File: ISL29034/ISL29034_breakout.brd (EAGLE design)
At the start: 15.2 x 11.2 mm, 2 parts

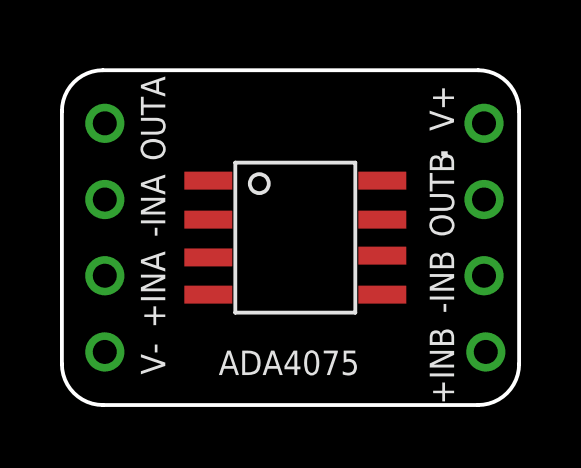
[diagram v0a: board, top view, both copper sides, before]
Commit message: Update new meme.
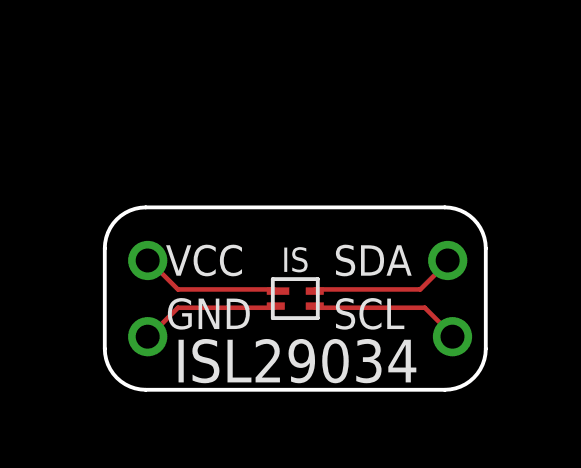
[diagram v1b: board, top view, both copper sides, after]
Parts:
- removed .: ADA4075, FaBo-Opamp:SOIC(NARROW)-8
- removed U$3: 8PIN, FaBo-Breakout:8PIN
- added IS: IN-ISL29034, FaBo-Mems:INTERSIL-ISL29034
- added U$1: 4PIN, FaBo-Breakout:4PIN
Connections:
- removed net 1: ..1, U$3.1
- removed net 2: ..2, U$3.2
- removed net 3: ..3, U$3.3
- removed net 4: ..4, U$3.4
- removed net 5: ..5, U$3.5
- removed net 6: ..6, U$3.6
- removed net 7: ..7, U$3.7
- removed net 8: ..8, U$3.8
- new net GND: IS.2, U$1.2
- new net SCL: IS.3, U$1.3
- new net SDA: IS.4, U$1.4
- new net VCC: IS.1, U$1.1
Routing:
- net SCL: track 0.00 -> 5.06 mm
- net SDA: track 0.00 -> 4.90 mm
- net VCC: track 0.00 -> 4.75 mm
- net GND: track 0.00 -> 4.68 mm
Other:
- board size 15.2 x 11.2 mm -> 12.7 x 6.1 mm
- board text added: "GND"
- board text added: "ISL29034"
- board text added: "SCL"
- board text added: "SDA"
- board text added: "VCC"
- board text removed: "+INA"
- board text removed: "+INB"
- board text removed: "-INA"
- board text removed: "-INB"
- board text removed: "ADA4075"
- board text removed: "OUTA"
- board text removed: "OUTB"
- board text removed: "V+"
- board text removed: "V-"
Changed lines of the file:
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@@
 <setting verticaltext="up"/>
 </settings>
-<grid distance="0.25" unitdist="mm" unit="mm" style="lines" multiple="1" display="yes" altdistance="0.025" altunitdist="inch" altunit="inch"/>
+<grid distance="0.01" unitdist="inch" unit="inch" style="lines" multiple="1" display="no" altdistance="0.025" altunitdist="inch" altunit="inch"/>
 <layers>
 <layer number="1" name="Top" color="4" fill="1" visible="yes" active="yes"/>
@@
 <layer number="49" name="Reference" color="7" fill="1" visible="yes" active="yes"/>
 <layer number="50" name="dxf" color="7" fill="1" visible="no" active="no"/>
-<layer number="51" name="tDocu" color="14" fill="1" visible="yes" active="yes"/>
+<layer number="51" name="tDocu" color="7" fill="1" visible="yes" active="yes"/>
 <layer number="52" name="bDocu" color="7" fill="1" visible="yes" active="yes"/>
 <layer number="53" name="tGND_GNDA" color="7" fill="9" visible="no" active="no"/>
@@
 <layer number="154" name="FabDoc2" color="2" fill="1" visible="no" active="no"/>
 <layer number="155" name="FabDoc3" color="7" fill="15" visible="no" active="no"/>
-<layer number="160" name="O_Dim" color="12" fill="11" visible="yes" active="yes"/>
 <layer number="199" name="Contour" color="7" fill="1" visible="yes" active="yes"/>
-<layer number="200" name="200bmp" color="1" fill="10" visible="yes" active="yes"/>
+<layer number="200" name="200bmp" color="1" fill="10" visible="no" active="yes"/>
 <layer number="201" name="201bmp" color="2" fill="1" visible="no" active="no"/>
 <layer number="202" name="202bmp" color="3" fill="1" visible="no" active="no"/>
@@
 <board>
 <plain>
-<text x="3.794" y="1.262" size="0.8128" layer="21">ADA4075</text>
-<text x="2.016" y="8.398" size="0.8128" layer="21" rot="R90">OUTA</text>
-<text x="2.016" y="5.858" size="0.8128" layer="21" rot="R90">-INA</text>
-<text x="2.016" y="2.818" size="0.8128" layer="21" rot="R90">+INA</text>
-<text x="11.64" y="9.398" size="0.8128" layer="21" rot="R90">V+</text>
-<text x="11.644" y="5.858" size="0.8128" layer="21" rot="R90">OUTB</text>
-<text x="11.644" y="3.318" size="0.8128" layer="21" rot="R90">-INB</text>
-<text x="11.644" y="0.278" size="0.8128" layer="21" rot="R90">+INB</text>
-<text x="2.016" y="1.278" size="0.8128" layer="21" rot="R90">V-</text>
+<text x="2.286" y="1.016" size="1.4224" layer="21">ISL29034</text>
+<text x="2.032" y="4.572" size="1.016" layer="21">VCC</text>
+<text x="2.032" y="2.794" size="1.016" layer="21">GND</text>
+<text x="7.62" y="4.572" size="1.016" layer="21">SDA</text>
+<text x="7.62" y="2.794" size="1.016" layer="21">SCL</text>
 </plain>
 <attributes>
@@
 </class>
 </classes>
-<designrules name="Elecrow_2-layer_eagle_rule">
+<designrules name="SeeedStudio_2layer_DRU_no_angle_20140221">
 <description language="de">&lt;b&gt;EAGLE Design Rules&lt;/b&gt;
 &lt;p&gt;
@@
 necessary adjustments and save your customized
 design rules under a new name.</description>
-<description language="zh">&lt;b&gt;Elecrow EAGLE Design Rules&lt;/b&gt;
+<description language="zh">&lt;b&gt;Seeed Studio EAGLE Design Rules&lt;/b&gt;
 </description>
 <param name="layerSetup" value="(1*16)"/>
-<param name="mtCopper" value="0.035mm 0.035mm 0.035mm 0.035mm 0.035mm 0.035mm 0.035mm 0.035mm 0.035mm 0.035mm 0.035mm 0.035mm 0.035mm 0.035mm 0.035mm 0.035mm"/>
-<param name="mtIsolate" value="1.5mm 0.15mm 0.2mm 0.15mm 0.2mm 0.15mm 0.2mm 0.15mm 0.2mm 0.15mm 0.2mm 0.15mm 0.2mm 0.15mm 0.2mm"/>
+<param name="mtCopper" value="0.035mm 0.0175mm 0.035mm 0.035mm 0.035mm 0.035mm 0.035mm 0.035mm 0.035mm 0.035mm 0.035mm 0.035mm 0.035mm 0.035mm 0.0175mm 0.035mm"/>
+<param name="mtIsolate" value="1.5mm 1.1mm 0.2mm 0.15mm 0.2mm 0.15mm 0.2mm 0.15mm 0.2mm 0.15mm 0.2mm 0.15mm 0.2mm 0.15mm 0.2mm"/>
 <param name="mdWireWire" value="6mil"/>
 <param name="mdWirePad" value="6mil"/>
@@
 </autorouter>
 <elements>
-<element name="U$3" library="FaBo-Breakout" package="8PIN" value="8PIN" x="7.46" y="5.842"/>
-<element name="." library="FaBo-Opamp" package="SOIC(NARROW)-8" value="ADA4075" x="6.35" y="5.842" rot="R270"/>
+<element name="U$1" library="FaBo-Breakout" package="4PIN" value="4PIN" x="6.35" y="3.81"/>
+<element name="IS" library="FaBo-Mems" package="INTERSIL-ISL29034" value="IN-ISL29034" x="6.35" y="3.81"/>
 </elements>
 <signals>
-<signal name="1">
-<contactref element="U$3" pad="1"/>
-<contactref element="." pad="1"/>
-<wire x1="3.45" y1="7.742" x2="0" y2="9.652" width="0" layer="19" extent="1-1"/>
+<signal name="VCC">
+<contactref element="U$1" pad="1"/>
+<contactref element="IS" pad="1"/>
+<wire x1="2.4384" y1="4.1148" x2="5.6388" y2="4.1148" width="0.1524" layer="1"/>
+<wire x1="1.524" y1="5.0292" x2="2.4384" y2="4.1148" width="0.1524" layer="1"/>
+<wire x1="5.6388" y1="4.1148" x2="5.775" y2="4.06" width="0.1524" layer="1"/>
+<wire x1="1.524" y1="5.0292" x2="1.43" y2="5.08" width="0.1524" layer="1"/>
 </signal>
-<signal name="2">
-<contactref element="U$3" pad="2"/>
-<contactref element="." pad="2"/>
-<wire x1="0" y1="7.112" x2="3.45" y2="6.442" width="0" layer="19" extent="1-1"/>
+<signal name="GND">
+<contactref element="U$1" pad="2"/>
+<contactref element="IS" pad="2"/>
+<wire x1="2.4384" y1="3.5052" x2="5.6388" y2="3.5052" width="0.1524" layer="1"/>
+<wire x1="1.524" y1="2.5908" x2="2.4384" y2="3.5052" width="0.1524" layer="1"/>
+<wire x1="5.6388" y1="3.5052" x2="5.7" y2="3.56" width="0.1524" layer="1"/>
+<wire x1="1.524" y1="2.5908" x2="1.43" y2="2.54" width="0.1524" layer="1"/>
 </signal>
-<signal name="3">
-<contactref element="U$3" pad="3"/>
-<contactref element="." pad="3"/>
-<wire x1="0" y1="4.572" x2="3.45" y2="5.182" width="0" layer="19" extent="1-1"/>
+<signal name="SDA">
+<contactref element="U$1" pad="4"/>
+<contactref element="IS" pad="4"/>
+<wire x1="10.5156" y1="4.1148" x2="7.0104" y2="4.1148" width="0.1524" layer="1"/>
+<wire x1="11.43" y1="5.0292" x2="10.5156" y2="4.1148" width="0.1524" layer="1"/>
+<wire x1="7.0104" y1="4.1148" x2="7" y2="4.06" width="0.1524" layer="1"/>
+<wire x1="11.43" y1="5.0292" x2="11.43" y2="5.08" width="0.1524" layer="1"/>
 </signal>
-<signal name="4">
-<contactref element="U$3" pad="4"/>
-<contactref element="." pad="4"/>
-<wire x1="0" y1="2.032" x2="3.45" y2="3.942" width="0" layer="19" extent="1-1"/>
-</signal>
-<signal name="8">
-<contactref element="U$3" pad="8"/>
-<contactref element="." pad="8"/>
-<wire x1="9.25" y1="7.742" x2="12.64" y2="9.652" width="0" layer="19" extent="1-1"/>
-</signal>
-<signal name="7">
-<contactref element="U$3" pad="7"/>
-<contactref element="." pad="7"/>
-<wire x1="9.25" y1="6.442" x2="12.64" y2="7.112" width="0" layer="19" extent="1-1"/>
-</signal>
-<signal name="6">
-<contactref element="U$3" pad="6"/>
-<contactref element="." pad="6"/>
-<wire x1="9.25" y1="5.242" x2="12.64" y2="4.572" width="0" layer="19" extent="1-1"/>
-</signal>
-<signal name="5">
-<contactref element="U$3" pad="5"/>
-<contactref element="." pad="5"/>
-<wire x1="12.7" y1="2.032" x2="9.25" y2="3.942" width="0" layer="19" extent="1-1"/>
+<signal name="SCL">
+<contactref element="IS" pad="3"/>
+<contactref element="U$1" pad="3"/>
+<wire x1="10.668" y1="3.5052" x2="7.0104" y2="3.5052" width="0.1524" layer="1"/>
+<wire x1="11.5824" y1="2.5908" x2="10.668" y2="3.5052" width="0.1524" layer="1"/>
+<wire x1="7.0104" y1="3.5052" x2="7" y2="3.56" width="0.1524" layer="1"/>
+<wire x1="11.5824" y1="2.5908" x2="11.59" y2="2.54" width="0.1524" layer="1"/>
 </signal>
 </signals>
-<errors>
-</errors>
 </board>
 </drawing>
